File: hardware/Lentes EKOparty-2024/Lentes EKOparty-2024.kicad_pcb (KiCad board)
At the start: 2 copper layers, 43.8 x 8.6 mm, 3 parts

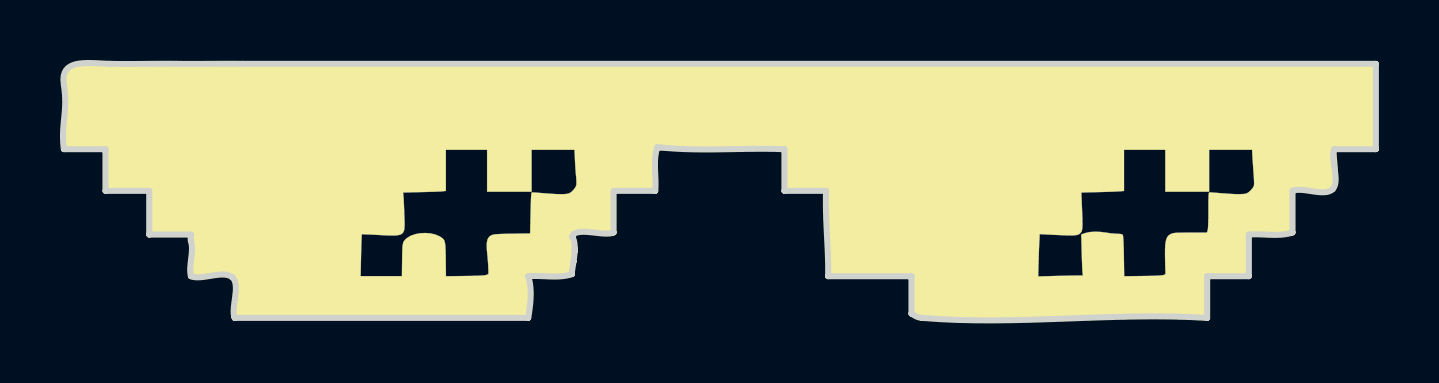
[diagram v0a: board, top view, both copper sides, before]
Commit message: feat(Hw): Update lentes
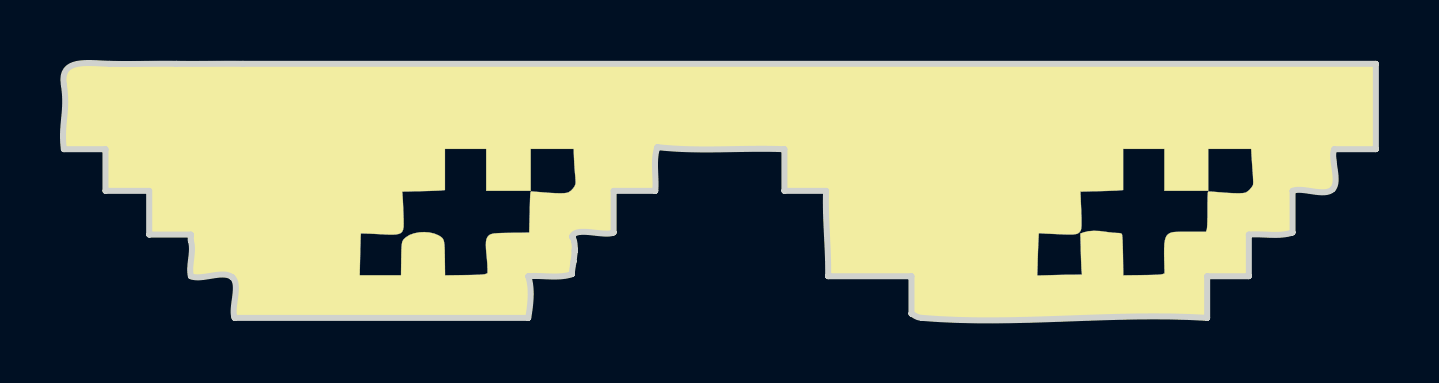
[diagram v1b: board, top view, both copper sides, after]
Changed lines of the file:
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@@
 	(footprint "Eko2024:llama-2-flaca"
 		(layer "F.Cu")
-		(at 129.02 64.96)
+		(at 128.99 64.93)
 		(property "Reference" "Ref**"
 			(at 0 0 0)
@@
 	(footprint "Eko2024:llama intermedia_Contorno"
 		(layer "F.Cu")
-		(at 129.01 64.95)
+		(at 129 64.93)
 		(property "Reference" "Ref**"
 			(at 0 0 0)
@@
 		(net 0)
 		(net_name "")
-		(layer "Edge.Cuts")
+		(layers "F&B.Cu")
 		(hatch edge 0.5)
 		(connect_pads
@@
 		(filled_areas_thickness no)
 		(keepout
-			(tracks not_allowed)
-			(vias not_allowed)
-			(pads not_allowed)
+			(tracks allowed)
+			(vias allowed)
+			(pads allowed)
 			(copperpour not_allowed)
 			(footprints allowed)
@@
 		(polygon
 			(pts
-				(xy 107.13 60.71) (xy 150.855558 60.697123) (xy 150.88 69.38) (xy 107.12 69.38) (xy 107.1 60.7)
-			)
-		)
+				(xy 146.96 63.3) (xy 142.16 63.29) (xy 142.16 64.76) (xy 140.87 64.76) (xy 140.86 66.15) (xy 139.28 66.2)
+				(xy 139.29 67.9) (xy 144.15 67.94) (xy 144.16 66.53) (xy 145.39 66.52) (xy 145.41 65.23) (xy 146.96 65.24)
+			)
+		)
+	)
+	(zone
+		(net 0)
+		(net_name "")
+		(layers "F&B.Cu")
+		(hatch edge 0.5)
+		(connect_pads
+			(clearance 0)
+		)
+		(min_thickness 0.25)
+		(filled_areas_thickness no)
+		(keepout
+			(tracks allowed)
+			(vias allowed)
+			(pads allowed)
+			(copperpour not_allowed)
+			(footprints allowed)
+		)
+		(fill
+			(thermal_gap 0.5)
+			(thermal_bridge_width 0.5)
+		)
+		(polygon
+			(pts
+				(xy 124.33 63.35) (xy 119.37 63.33) (xy 119.32 64.67) (xy 118.1 64.7) (xy 118 66.15) (xy 116.25 66.1)
+				(xy 116.26 68.05) (xy 121.78 68.03) (xy 121.78 66.58) (xy 123.01 66.58) (xy 123.06 65.29) (xy 124.33 65.24)
+			)
+		)
